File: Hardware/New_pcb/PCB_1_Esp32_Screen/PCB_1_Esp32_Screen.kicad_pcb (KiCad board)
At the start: 2 copper layers, 77.5 x 62 mm, 3 parts, among them J1 Conn_01x12_Pin, J2 Conn_01x07_Pin

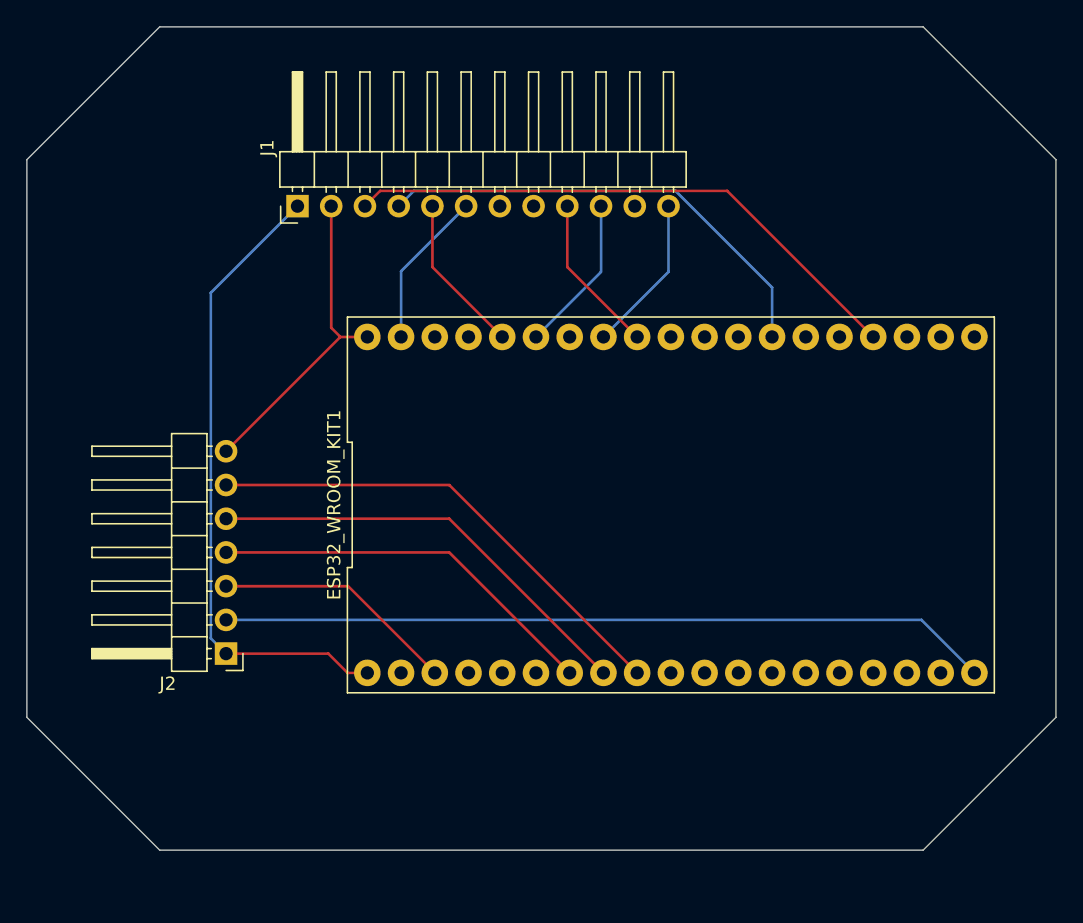
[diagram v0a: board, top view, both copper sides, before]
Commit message: pcb amelioration
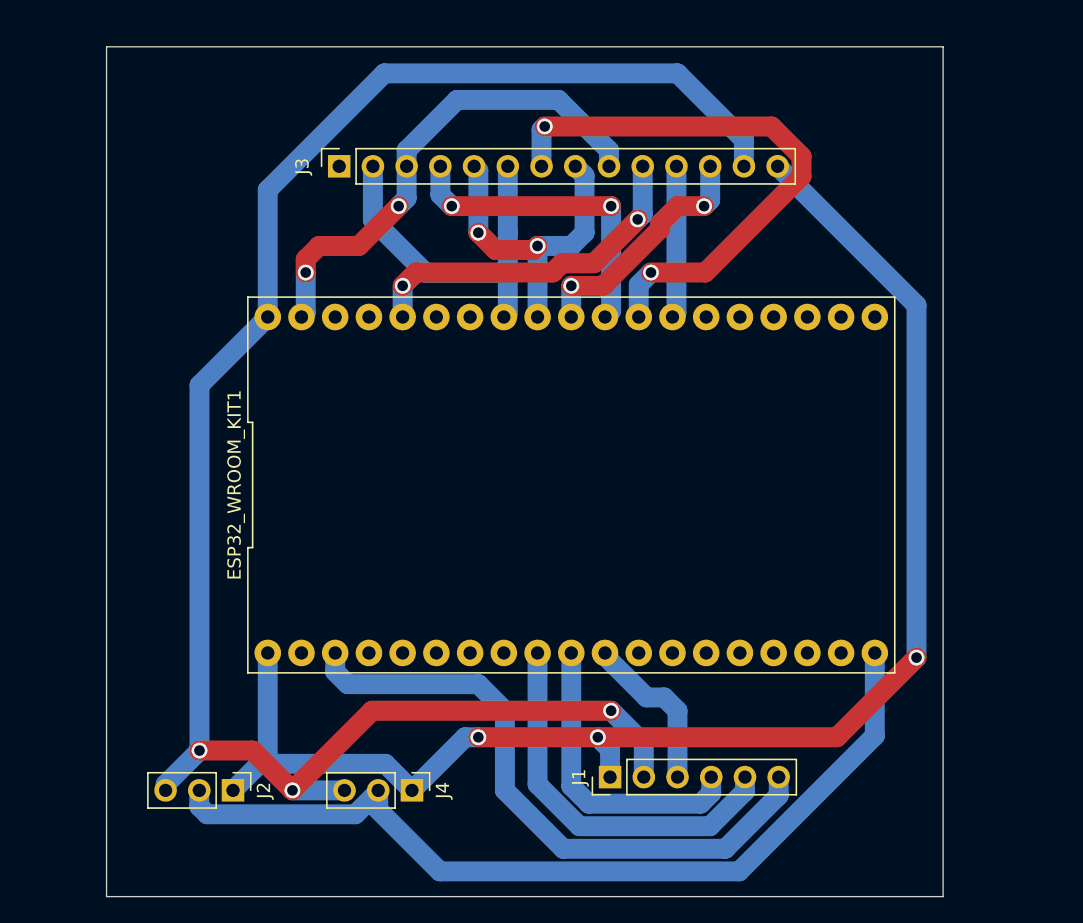
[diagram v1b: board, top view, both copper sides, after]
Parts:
- added J3: Conn_01x14_Socket, Connector_PinSocket_2.54mm:PinSocket_1x14_P2.54mm_Vertical, F.Cu at (118.5, 78.0)
- added J4: Conn_01x03_Pin, Connector_PinHeader_2.54mm:PinHeader_1x03_P2.54mm_Vertical, F.Cu at (124.0, 125.0)
- J1: value Conn_01x12_Pin -> Conn_01x06_Pin; footprint Connector_PinHeader_2.54mm:PinHeader_1x12_P2.54mm_Horizontal -> Connector_PinHeader_2.54mm:PinHeader_1x06_P2.54mm_Vertical
- J2: value Conn_01x07_Pin -> Conn_01x03_Pin; footprint Connector_PinHeader_2.54mm:PinHeader_1x07_P2.54mm_Horizontal -> Connector_PinHeader_2.54mm:PinHeader_1x03_P2.54mm_Vertical
- moved J1 49.0 mm to (138.9, 124.0)
- moved J2 10.3 mm to (110.5, 125.0), turned to -90 degrees
- moved ESP32_WROOM_KIT1 7.65 mm to (136.0, 102.0)
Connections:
- ESP32_WROOM_KIT1 pad 10: unconnected-(ESP32_WROOM_KIT1-GPIO26-Pad10) -> Clock
- ESP32_WROOM_KIT1 pad 11: unconnected-(ESP32_WROOM_KIT1-GPIO27-Pad11) -> Trig
- ESP32_WROOM_KIT1 pad 23: Net-(ESP32_WROOM_KIT1-GPIO15) -> unconnected-(ESP32_WROOM_KIT1-GPIO15-Pad23)
- ESP32_WROOM_KIT1 pad 26: Net-(ESP32_WROOM_KIT1-GPIO4) -> RESET
- ESP32_WROOM_KIT1 pad 27: unconnected-(ESP32_WROOM_KIT1-GPIO16-Pad27) -> LED
- ESP32_WROOM_KIT1 pad 28: unconnected-(ESP32_WROOM_KIT1-GPIO17-Pad28) -> T_CS
- ESP32_WROOM_KIT1 pad 29: unconnected-(ESP32_WROOM_KIT1-GPIO5-Pad29) -> CS
- ESP32_WROOM_KIT1 pad 30: Net-(ESP32_WROOM_KIT1-GPIO18) -> SCK
- ESP32_WROOM_KIT1 pad 31: Net-(ESP32_WROOM_KIT1-GPIO19) -> MISO
- ESP32_WROOM_KIT1 pad 33: Net-(ESP32_WROOM_KIT1-GPIO21) -> unconnected-(ESP32_WROOM_KIT1-GPIO21-Pad33)
- ESP32_WROOM_KIT1 pad 34: Net-(ESP32_WROOM_KIT1-GPIO2) -> DC
- ESP32_WROOM_KIT1 pad 37: Net-(ESP32_WROOM_KIT1-GPIO23) -> MOSI
- ESP32_WROOM_KIT1 pad 7: Data -> unconnected-(ESP32_WROOM_KIT1-GPIO32-Pad7)
- ESP32_WROOM_KIT1 pad 8: Clock -> unconnected-(ESP32_WROOM_KIT1-GPIO33-Pad8)
- ESP32_WROOM_KIT1 pad 9: Trig -> Data
- J1 pad 3: Net-(ESP32_WROOM_KIT1-GPIO15) -> Trig
- J1 pad 4: Net-(ESP32_WROOM_KIT1-GPIO4) -> Clock
- J1 pad 5: Net-(ESP32_WROOM_KIT1-GPIO2) -> Data
- J1 pad 6: Net-(ESP32_WROOM_KIT1-GPIO23) -> Analog_Pin1
- J2 pad 3: Analog_Pin1 -> GND
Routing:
- net GND: track 24.3 -> 136.6 mm, vias 0 -> 3
- net +3.3V: track 48.1 -> 110.6 mm, vias 0 -> 3
- net Net-(ESP32_WROOM_KIT1-GPIO15): track 43.3 -> 0.00 mm
- net LED: track 0.00 -> 42.9 mm, vias 0 -> 2
- net MOSI: track 0.00 -> 37.2 mm, vias 0 -> 2
- net Net-(ESP32_WROOM_KIT1-GPIO4): track 35.3 -> 0.00 mm
- net Analog_Pin1: track 18.4 -> 46.9 mm
- net MISO: track 0.00 -> 27.3 mm
- net DC: track 0.00 -> 26.3 mm, vias 0 -> 2
- net SCK: track 0.00 -> 24.8 mm, vias 0 -> 2
- net Trig: track 36.8 -> 12.4 mm
- net T_CS: track 0.00 -> 23.9 mm, vias 0 -> 2
- net CS: track 0.00 -> 18.3 mm, vias 0 -> 2
- net Net-(ESP32_WROOM_KIT1-GPIO18): track 12.0 -> 0.00 mm
- net Net-(ESP32_WROOM_KIT1-GPIO2): track 12.0 -> 0.00 mm
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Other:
- board size 77.5 x 62 mm -> 63 x 64 mm
